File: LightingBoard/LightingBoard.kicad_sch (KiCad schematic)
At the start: 27 parts, among them J1 Barrel_Jack_Switch, J4 Programming, J5 UART, J7 UART, U1 AVR32DD28-I/STX, U10 XC6206P502MR, U5 MCP4725xxx-xCH, U6 MCP4725xxx-xCH, X1 XRCGB32M000F1S2KR0

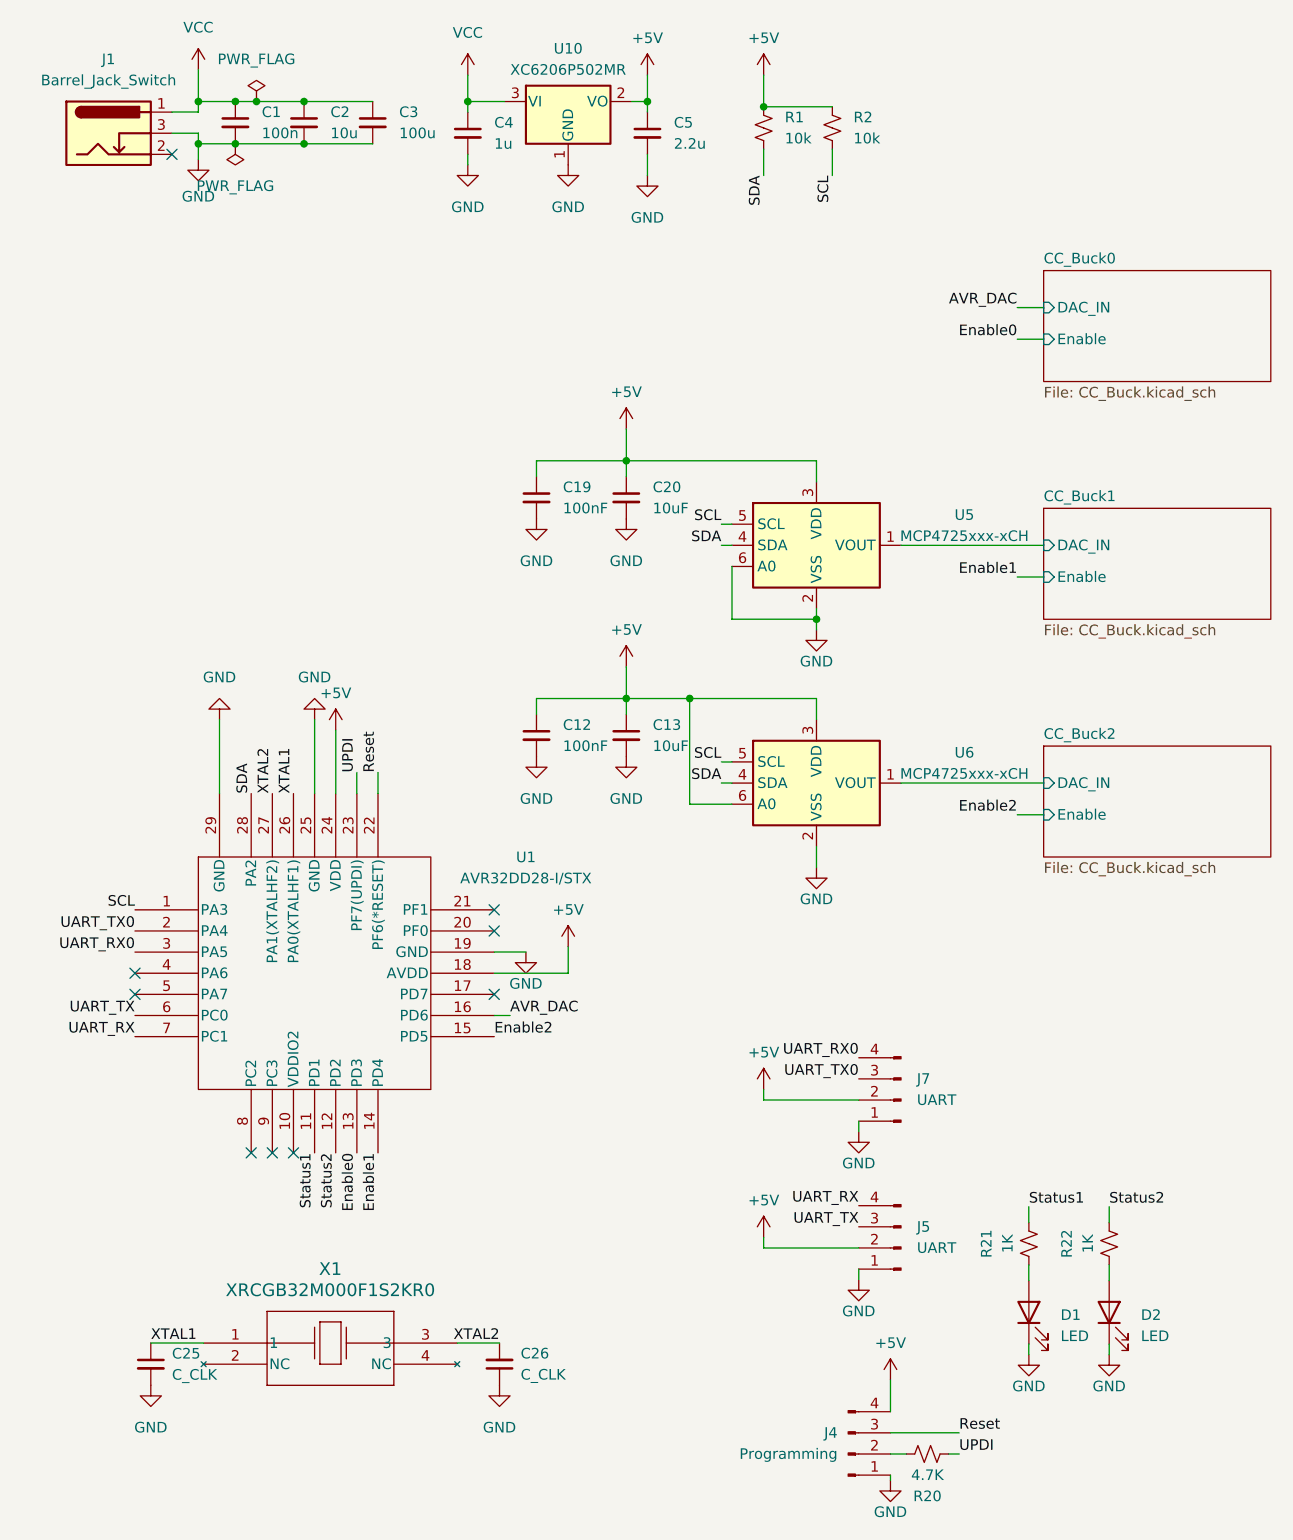
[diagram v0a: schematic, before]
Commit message: imma subsheet into your sheets
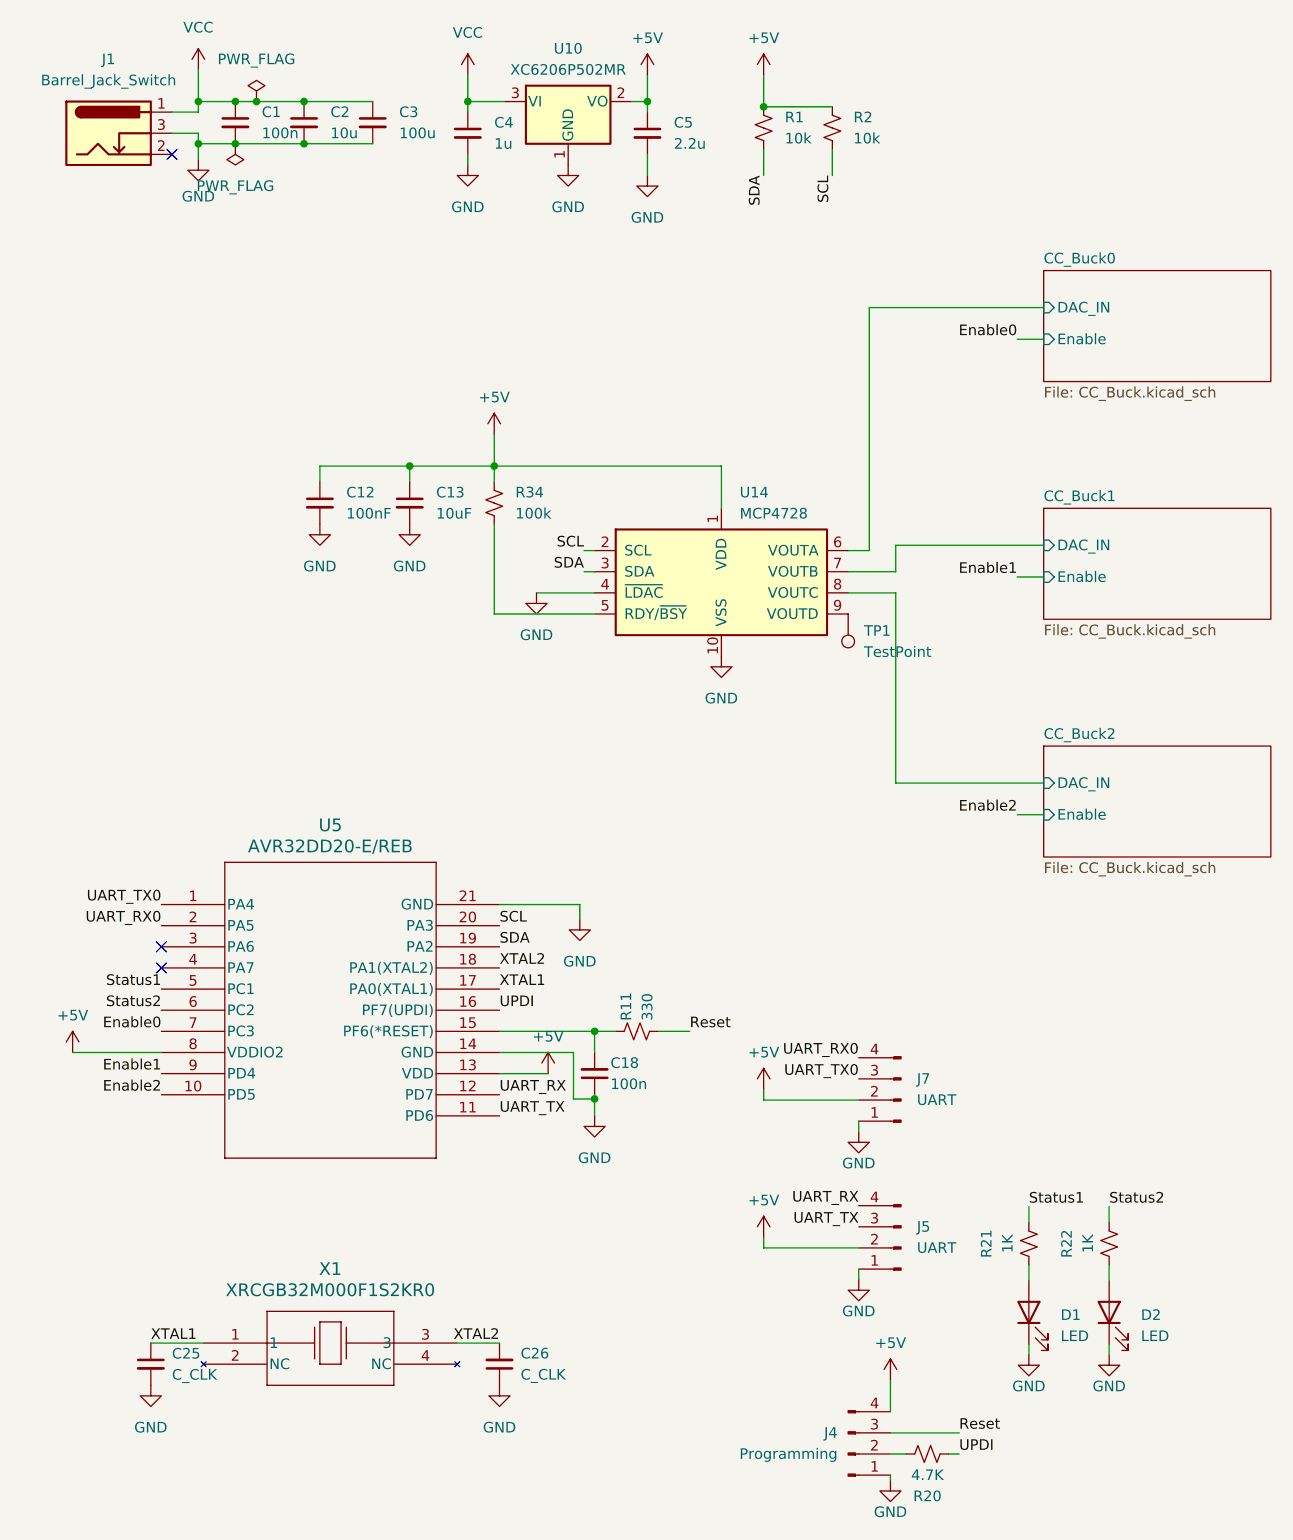
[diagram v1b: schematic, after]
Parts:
- removed C19: 100nF, Capacitor_SMD:C_0603_1608Metric, symbol Device:C_Small
- removed C20: 10uF, Capacitor_SMD:C_0603_1608Metric, symbol Device:C_Small
- removed U1: AVR32DD28-I/STX, Package_DFN_QFN:VQFN-28-1EP_4x4mm_P0.45mm_EP2.4x2.4mm, symbol CustomSymbols:AVR32DD28-I_STX
- removed U5, U6: MCP4725xxx-xCH, Package_TO_SOT_SMD:SOT-23-6, symbol Analog_DAC:MCP4725xxx-xCH
- added C18: 100n, Capacitor_SMD:C_0603_1608Metric, symbol Device:C_Small
- added R11: 330, Resistor_SMD:R_0603_1608Metric, symbol Device:R_Small_US
- added R34: 100k, Resistor_SMD:R_0603_1608Metric, symbol Device:R_Small_US
- added TP1: TestPoint, TestPoint:TestPoint_Pad_D1.0mm, symbol Connector:TestPoint
- added U14: MCP4728, Package_SO:MSOP-10_3x3mm_P0.5mm, symbol Analog_DAC:MCP4728
- added U5: AVR32DD20-E/REB, Package_DFN_QFN:VQFN-20-1EP_3x3mm_P0.4mm_EP1.7x1.7mm, symbol CustomSymbols:AVR32DD20-E_REB
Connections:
- net +5V: now also R34.1, U14.1 (VDD), U5.13 (VDD), U5.8 (VDDIO2)
- net CC_Buck1/DAC_IN: now also U14.7 (VOUTB)
- net CC_Buck2/DAC_IN: now also U14.8 (VOUTC)
- net Enable0: now also U5.7 (PC3)
- net Enable1: now also U5.9 (PD4)
- net Enable2: now also U5.10 (PD5)
- net GND: now also C18.1, U14.10 (VSS), U14.4 (~{LDAC}), U5.14 (GND), U5.21 (GND)
- net Reset: now also R11.1
- net SCL: now also U14.2 (SCL), U5.20 (PA3)
- net SDA: now also U14.3 (SDA), U5.19 (PA2)
- net Status1: now also U5.5 (PC1)
- net Status2: now also U5.6 (PC2)
- net UART_RX: now also U5.12 (PD7)
- net UART_RX0: now also U5.2 (PA5)
- net UART_TX: now also U5.11 (PD6)
- net UART_TX0: now also U5.1 (PA4)
- net UPDI: now also U5.16 (PF7(UPDI))
- net XTAL1: now also U5.17 (PA0(XTAL1))
- net XTAL2: now also U5.18 (PA1(XTAL2))
- new net: C18.2, R11.2, U5.15 (PF6(*RESET))
- new net: TP1.1, U14.9 (VOUTD)
- new net: R34.2, U14.5 (RDY/~{BSY})
- new net CC_Buck0/DAC_IN: U14.6 (VOUTA)
- no-connect marks 9 -> 3
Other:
- moved on the sheet: C12, C13
